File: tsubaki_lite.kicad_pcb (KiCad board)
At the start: 2 copper layers, 100 x 20 mm, 48 parts, among them J1 USB_C_Receptacle_USB2.0_16P, J2 Conn_01x02, J3 Conn_01x04, Q1 AO3400A, Q2 AO3400A, Q3 AO3400A, Q4 AO3400A, SW1 SW_SPST, SW2 SW_SPST, SW3 EC12E1240406, U1 CH32X033F8P6

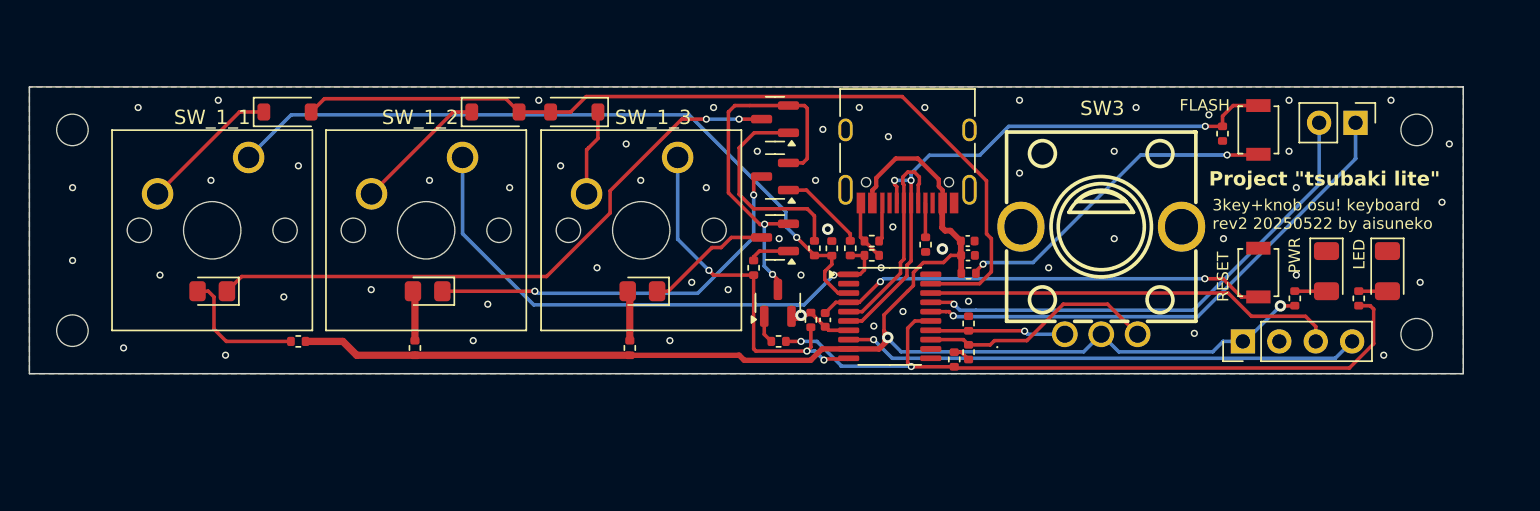
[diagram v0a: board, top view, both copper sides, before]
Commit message: rev3
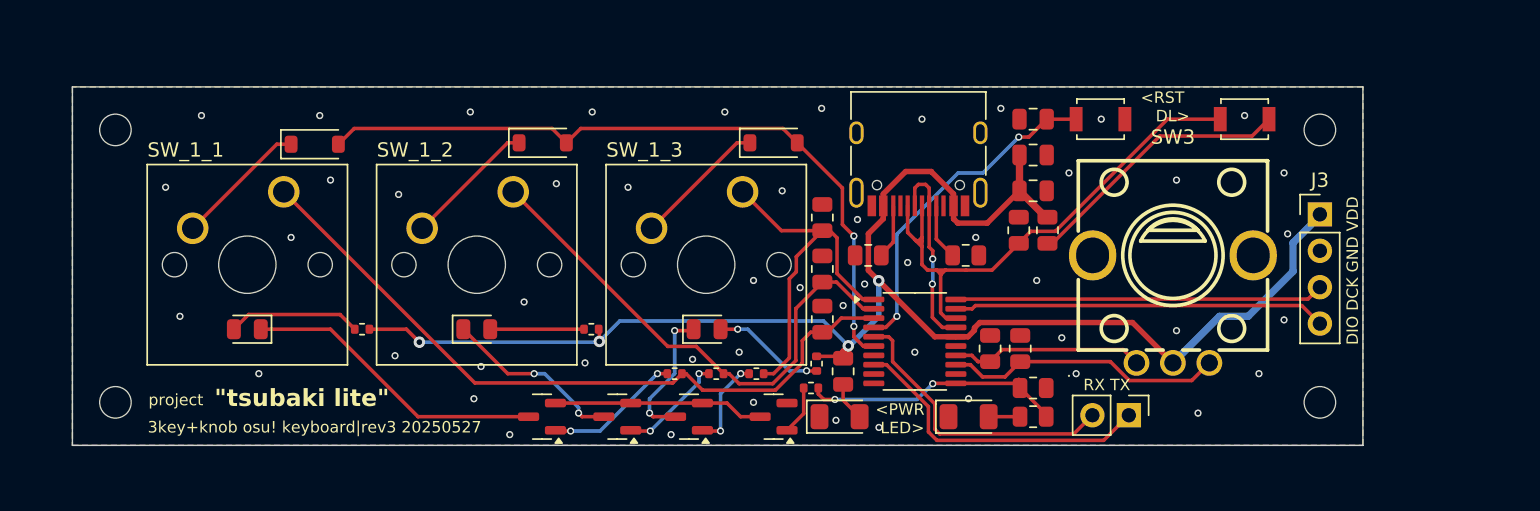
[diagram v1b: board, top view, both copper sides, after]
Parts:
- C1, C2, C3: footprint Capacitor_SMD:C_0402_1005Metric -> Capacitor_SMD:C_0805_2012Metric
- L_1_1, L_1_2, L_1_3: footprint LED_SMD:LED_0805_2012Metric_Pad1.15x1.40mm_HandSolder -> LED_SMD:LED_0805_2012Metric
- R1, R10, R12, R14, R15, R16, R2, R3, R4, R5, R7, R8: footprint Resistor_SMD:R_0402_1005Metric -> Resistor_SMD:R_0805_2012Metric
- SW3: footprint ProjectLocal:SW-TH_EC12E1240406 -> local:SW-TH_EC12E1240406
- U1: value CH32X033F8P6 -> CH32X035F7P6
- moved D2 35.4 mm to (149.5, 113.0), turned to 0 degrees
- moved R5 31.9 mm to (149.8, 109.8), turned to -90 degrees
- moved D1 30.9 mm to (158.5, 113.0), turned to 0 degrees
- moved Q1 26.4 mm to (128.8, 113.0)
- moved J2 25.8 mm to (169.7, 112.9)
- moved R4 24.2 mm to (163.0, 113.0), turned to 180 degrees
- moved C1 20.2 mm to (163.0, 92.2), turned to 180 degrees
- moved Q2 20.0 mm to (134.0, 113.0)
- moved R16 15.7 mm to (162.0, 100.0), turned to -90 degrees
- moved SW1 15.4 mm to (167.7, 92.2), turned to 0 degrees
- moved D_1_3 14.1 mm to (144.9, 93.9), turned to 0 degrees
- moved Q3 13.9 mm to (139.0, 113.0)
- moved R6 13.1 mm to (138.0, 110.0), turned to 180 degrees
- moved R_1_3 13.1 mm to (147.9, 109.3), turned to -90 degrees
- moved R9 12.8 mm to (140.9, 110.0), turned to 180 degrees
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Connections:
- U1 pad 1: /COL2 -> /COL3
- U1 pad 10: /COL3 -> unconnected-(U1-PA4-Pad10)
- U1 pad 11: unconnected-(U1-PA11-Pad11) -> /LED_CTRL
- U1 pad 15: /LED_CTRL -> GND
- U1 pad 16: /TX -> VDD
- U1 pad 17: /RX -> /DM
- U1 pad 18: /DCK -> /DP
- U1 pad 19: /ROW1 -> /DIO
- U1 pad 2: unconnected-(U1-PA7-Pad2) -> /COL2
- U1 pad 20: unconnected-(U1-PA5-Pad20) -> /DCK
- U1 pad 5: /DM -> /RX
- U1 pad 6: /DP -> /ROW1
- U1 pad 7: GND -> unconnected-(U1-PA1-Pad7)
- U1 pad 8: /DIO -> /TX
- U1 pad 9: VDD -> unconnected-(U1-PA3-Pad9)
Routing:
- net /LED_CTRL: track 50.6 -> 19.1 mm
- net Net-(L_1_1-K): track 43.2 -> 20.8 mm, vias 2 -> 0
- net Net-(L_1_2-K): track 28.2 -> 12.6 mm
- net /TX: track 36.9 -> 21.7 mm, vias 1 -> 0
- net /RX: track 35.3 -> 20.5 mm, vias 1 -> 0
- net /ROW1: track 61.8 -> 50.5 mm, vias 0 -> 2
- net Net-(Q1-S): track 26.4 -> 15.1 mm, vias 2 -> 0
- net VDD: track 98.7 -> 109.6 mm, vias 2 -> 4
- net /DIO: track 36.1 -> 26.0 mm, vias 1 -> 0
- net GND: track 9.74 -> 0.00 mm, vias 59 -> 51
- net /RESET: track 31.7 -> 23.5 mm
- net Net-(Q1-G): track 14.7 -> 9.93 mm, vias 0 -> 2
- net Net-(L_1_3-A): track 3.51 -> 7.91 mm, vias 0 -> 2
- net Net-(SW2-B): track 23.2 -> 19.0 mm, vias 2 -> 0
- net /DP: track 42.0 -> 38.3 mm, vias 3 -> 0
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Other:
- board size 100 x 20 mm -> 90 x 25 mm
- board text added: "3key+knob osu! keyboard|rev3 20250527"
- board text added: "<PWR LED>"
- board text added: "<RST DL>"
- board text added: "DIO DCK GND VDD"
- board text added: "project"
- board text added: "{dblquote}tsubaki lite{dblquote}"
- board text removed: "3key+knob osu! keyboard rev2 20250522 by aisuneko"
- board text removed: "FLASH"
- board text removed: "LED"
- board text removed: "PWR"
- board text removed: "Project {dblquote}tsubaki lite{dblquote}"
- board text removed: "RESET"
- board text removed: "VDD GND DCK DIO"
- board text removed: "wchlink"

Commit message: rev4
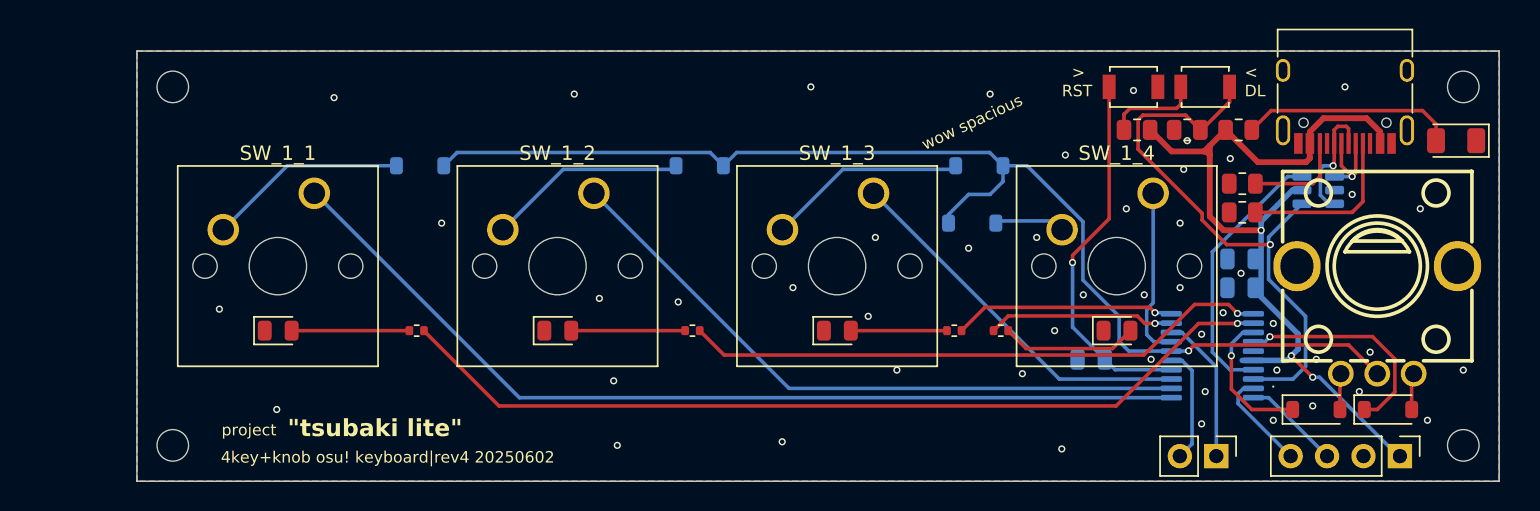
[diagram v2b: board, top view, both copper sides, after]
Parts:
- removed D2: LED, LED_SMD:LED_1206_3216Metric
- removed Q1, Q2, Q3, Q4: AO3400A, Package_TO_SOT_SMD:SOT-23
- removed R10, R12, R14, R15, R4, R7, R8: 10K, Resistor_SMD:R_0805_2012Metric
- removed R11, R13, R6, R9: 220R, Resistor_SMD:R_0402_1005Metric
- added D_1_4: 1N4148, Diode_SMD:D_SOD-123, B.Cu at (158.8, 99.5)
- added D_1_5: 1N4148, Diode_SMD:D_SOD-123, F.Cu at (182.8, 112.5)
- added D_1_6: 1N4148, Diode_SMD:D_SOD-123, F.Cu at (187.8, 112.5)
- added L_1_4: LED_Small, LED_SMD:LED_0805_2012Metric, F.Cu at (168.8, 107.0)
- added R_1_4: 560R, Resistor_SMD:R_0402_1005Metric, F.Cu at (160.8, 107.0)
- added SW_1_4: MX-compatible, Button_Switch_Keyboard:SW_Cherry_MX_1.00u_PCB, F.Cu at (171.4, 97.4)
- added U2: USBLC6-2SC6, Package_TO_SOT_SMD:SOT-23-6, B.Cu at (182.9, 97.2)
- C1, C2, C3, D_1_1, D_1_2, D_1_3, U1: moved to B.Cu
- moved H2 96.5 mm to (193.0, 90.0)
- moved H3 83.0 mm to (103.0, 115.0)
- moved D1 39.1 mm to (192.5, 93.8), turned to 180 degrees
- moved R5 32.3 mm to (177.3, 93.0), turned to 0 degrees
- moved J1 30.1 mm to (184.8, 89.9)
- moved R2 26.6 mm to (177.6, 96.8)
- moved U1 20.8 mm to (175.5, 108.8)
- moved R3 19.5 mm to (177.6, 98.8), turned to 180 degrees
- moved J3 17.8 mm to (188.6, 115.8), turned to -90 degrees
- moved C1 17.2 mm to (167.1, 109.0)
- moved C3 17.2 mm to (177.5, 104.0), turned to 180 degrees
- moved C2 15.3 mm to (177.5, 102.0), turned to 180 degrees
- moved D_1_3 14.4 mm to (159.2, 95.5)
- moved SW3 14.3 mm to (187.0, 106.3)
- moved R16 13.7 mm to (173.8, 93.0), turned to 0 degrees
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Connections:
- J1 pad A6: /DP -> Net-(J1-D+-PadA6)
- J1 pad A7: /DM -> Net-(J1-D--PadA7)
- J1 pad B6: /DP -> Net-(J1-D+-PadA6)
- J1 pad B7: /DM -> Net-(J1-D--PadA7)
- L_1_1 pad 1: Net-(L_1_1-K) -> GND
- L_1_2 pad 1: Net-(L_1_2-K) -> GND
- L_1_3 pad 1: Net-(L_1_3-K) -> GND
- R5 pad 2: Net-(D2-A) -> Net-(D1-A)
- R_1_1 pad 1: VDD -> /LED1
- R_1_2 pad 1: VDD -> /LED2
- R_1_3 pad 1: VDD -> /LED3
- SW3 pad A: /ROT_UP -> Net-(D_1_5-A)
- SW3 pad B: /ROT_DOWN -> Net-(D_1_6-A)
- SW3 pad C: VDD -> /ROW1
- U1 pad 1: /COL3 -> /COL1
- U1 pad 10: unconnected-(U1-PA4-Pad10) -> /LED3
- U1 pad 11: /LED_CTRL -> /LED2
- U1 pad 12: unconnected-(U1-PA6-Pad12) -> /LED1
- U1 pad 3: /COL1 -> /COL3
- U1 pad 7: unconnected-(U1-PA1-Pad7) -> /COL4
- U1 pad 9: unconnected-(U1-PA3-Pad9) -> /LED4
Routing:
- net /LED1: track 0.00 -> 62.4 mm, vias 0 -> 1
- net VDD: track 109.6 -> 59.6 mm, vias 4 -> 3
- net /LED2: track 0.00 -> 41.0 mm, vias 0 -> 1
- net /ROW1: track 50.5 -> 82.9 mm, vias 2 -> 1
- net Net-(L_1_1-K): track 20.8 -> 0.00 mm
- net /LED_CTRL: track 19.1 -> 0.00 mm, vias 2 -> 0
- net /DCK: track 25.7 -> 6.83 mm
- net /DIO: track 26.0 -> 7.09 mm
- net /LED3: track 0.00 -> 15.5 mm, vias 0 -> 1
- net /COL1: track 50.4 -> 65.7 mm
- net Net-(Q1-S): track 15.1 -> 0.00 mm
- net /LED4: track 0.00 -> 13.1 mm, vias 0 -> 1
- net Net-(D1-A): track 2.19 -> 15.0 mm
- net Net-(L_1_2-K): track 12.6 -> 0.00 mm, vias 2 -> 0
- net Net-(SW2-B): track 19.0 -> 6.55 mm
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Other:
- board size 90 x 25 mm -> 95 x 30 mm
- board text added: "4key+knob osu! keyboard|rev4 20250602"
- board text added: "< DL"
- board text added: "> RST"
- board text added: "wow spacious"
- board text removed: "3key+knob osu! keyboard|rev3 20250527"
- board text removed: "<PWR LED>"
- board text removed: "<RST DL>"
